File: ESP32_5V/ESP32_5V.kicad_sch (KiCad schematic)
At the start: 0 parts

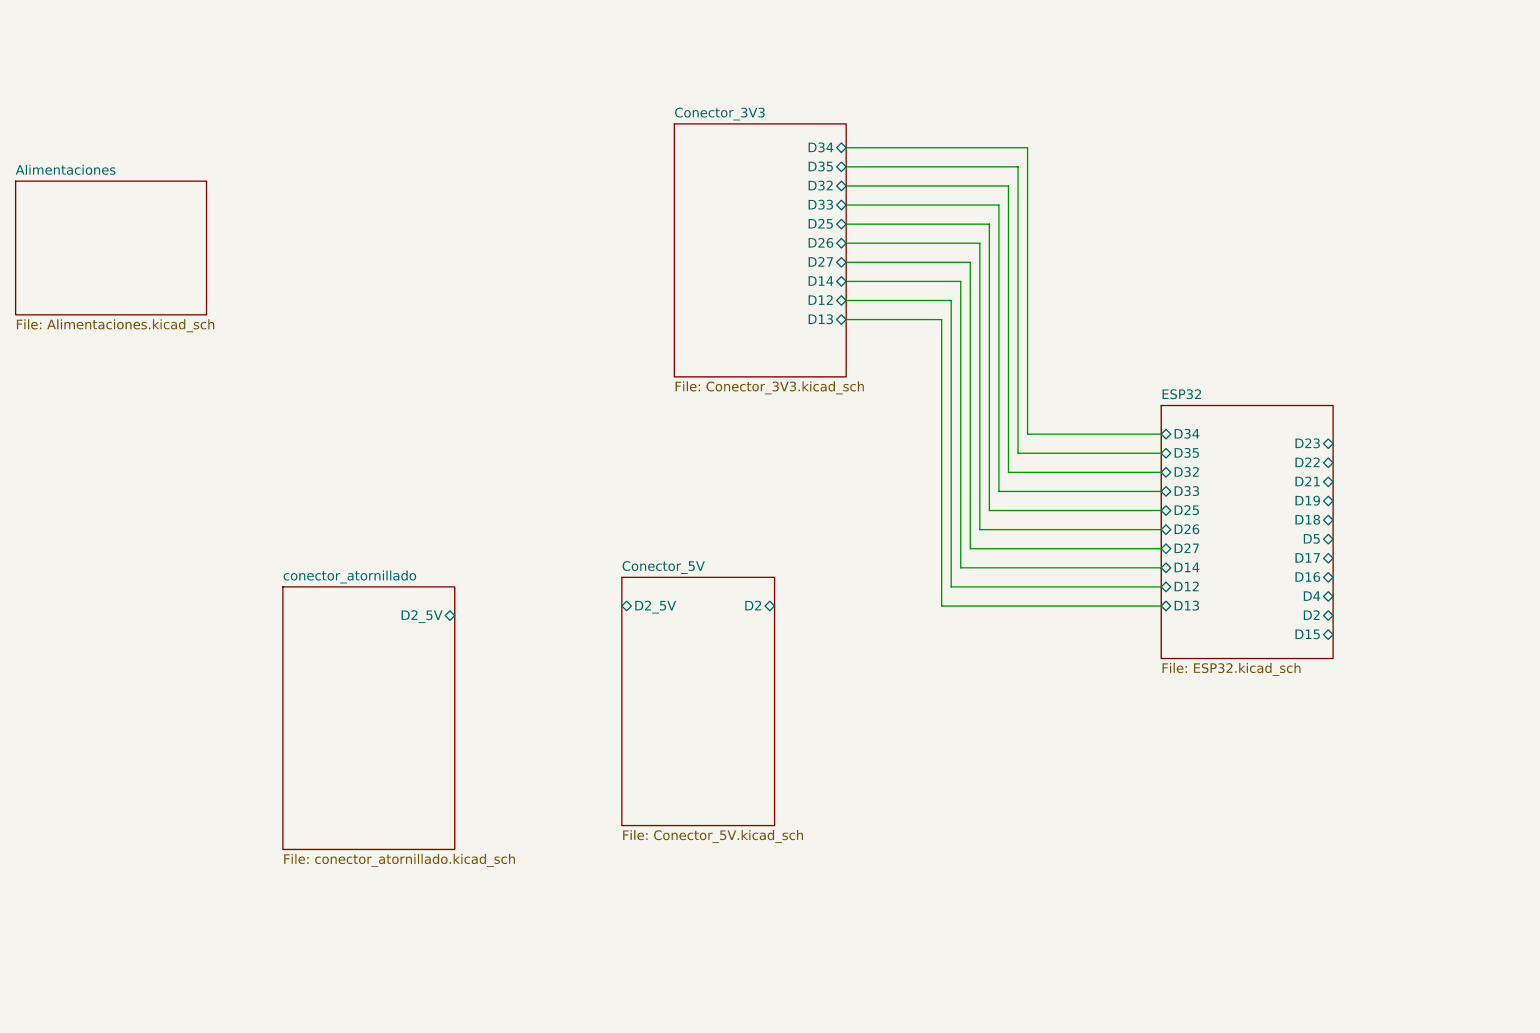
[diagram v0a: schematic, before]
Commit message: update
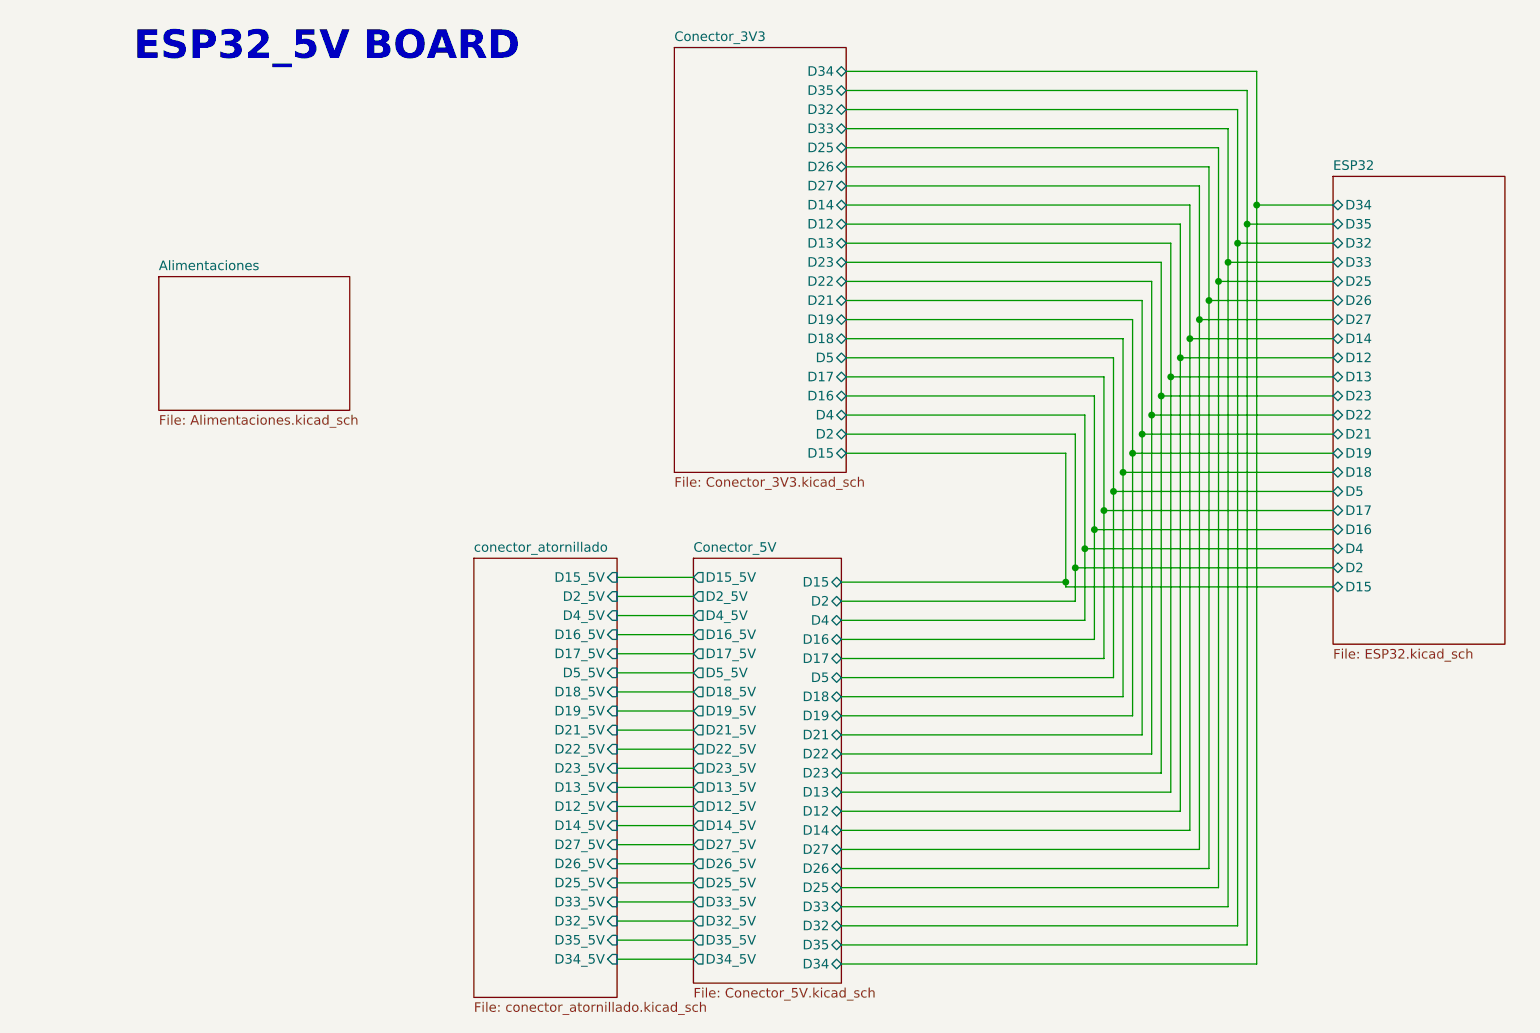
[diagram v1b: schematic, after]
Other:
- sheet Conector_3V3 ports: added D15, D16, D17, D18, D19, D2, D21, D22, D23, D4, D5; removed none
- sheet Conector_5V ports: added D12, D12_5V, D13, D13_5V, D14, D14_5V, D15, D15_5V, D16, D16_5V, D17, D17_5V, D18, D18_5V, D19, D19_5V, D21, D21_5V, D22, D22_5V, D23, D23_5V, D25, D25_5V, D26, D26_5V, D27, D27_5V, D32, D32_5V, D33, D33_5V, D34, D34_5V, D35, D35_5V, D4, D4_5V, D5, D5_5V; removed none
- sheet conector_atornillado ports: added D12_5V, D13_5V, D14_5V, D15_5V, D16_5V, D17_5V, D18_5V, D19_5V, D21_5V, D22_5V, D23_5V, D25_5V, D26_5V, D27_5V, D32_5V, D33_5V, D34_5V, D35_5V, D4_5V, D5_5V; removed none
- note added: "ESP32_5V BOARD"
